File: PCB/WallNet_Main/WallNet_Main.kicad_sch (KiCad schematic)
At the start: 29 parts, among them J1 Conn_01x05_Pin, SW1 SW, U1 BT832

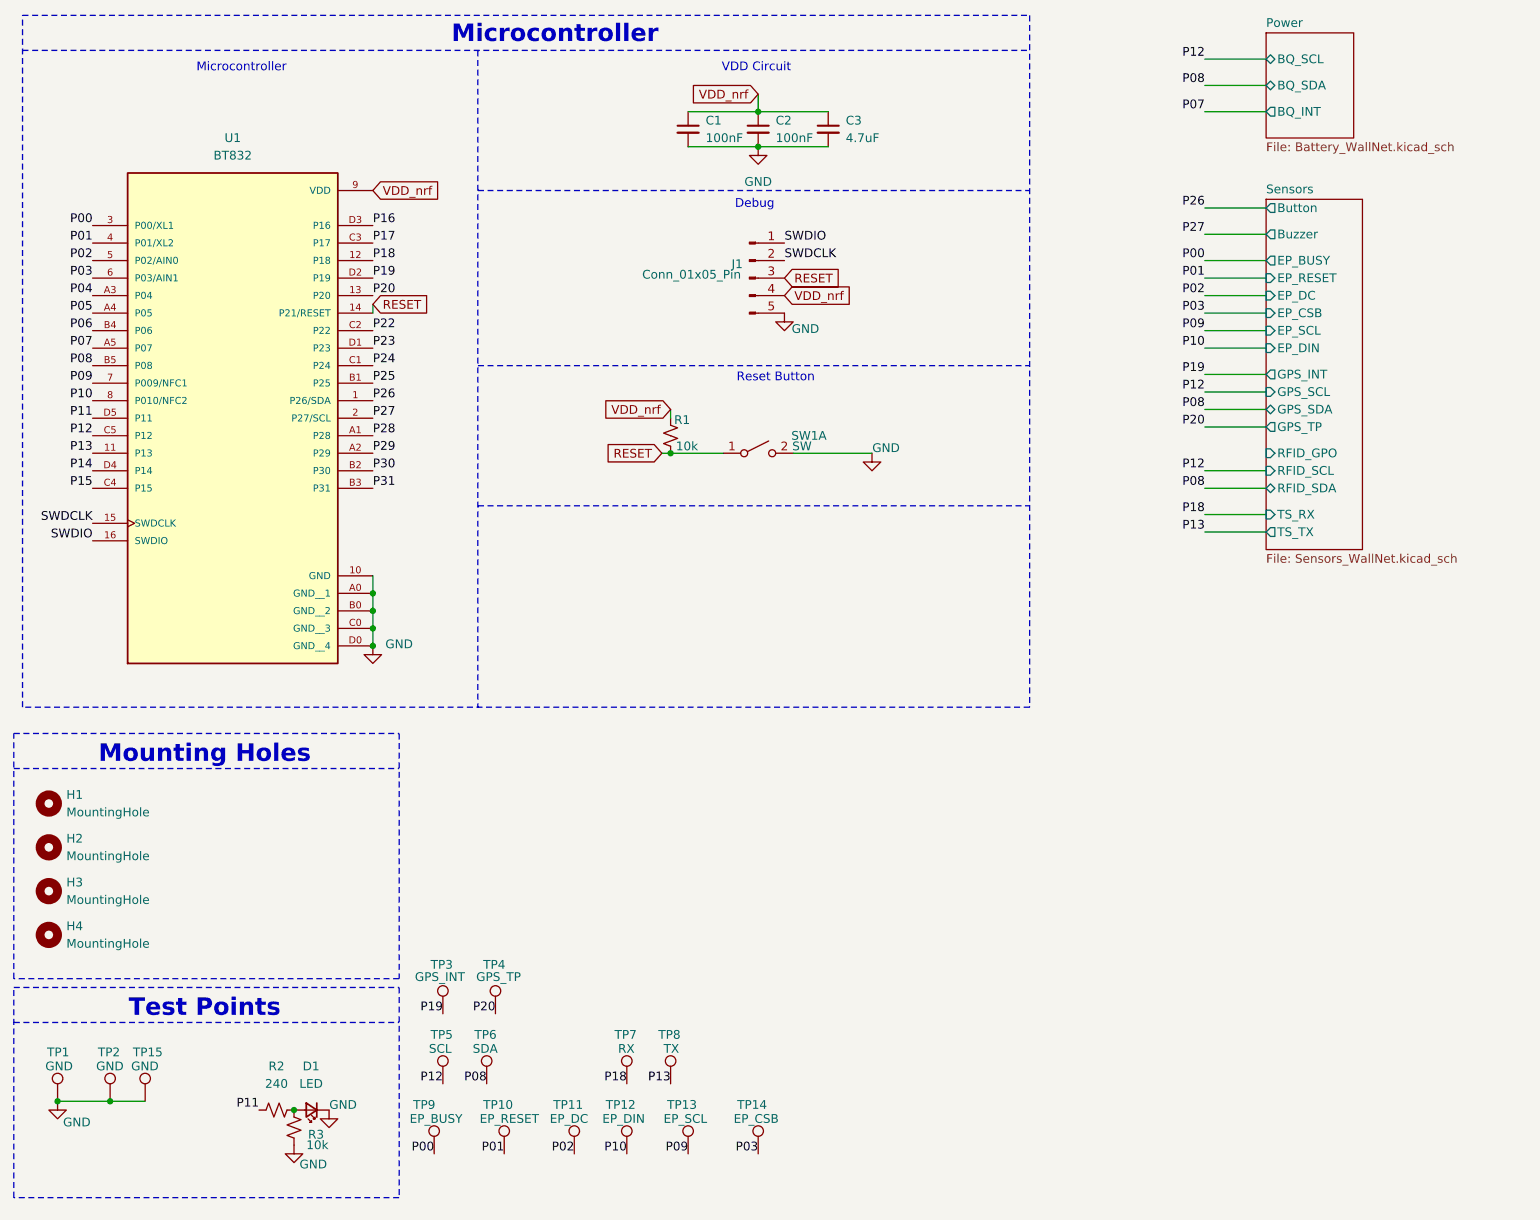
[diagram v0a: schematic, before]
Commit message: Implemented most changes
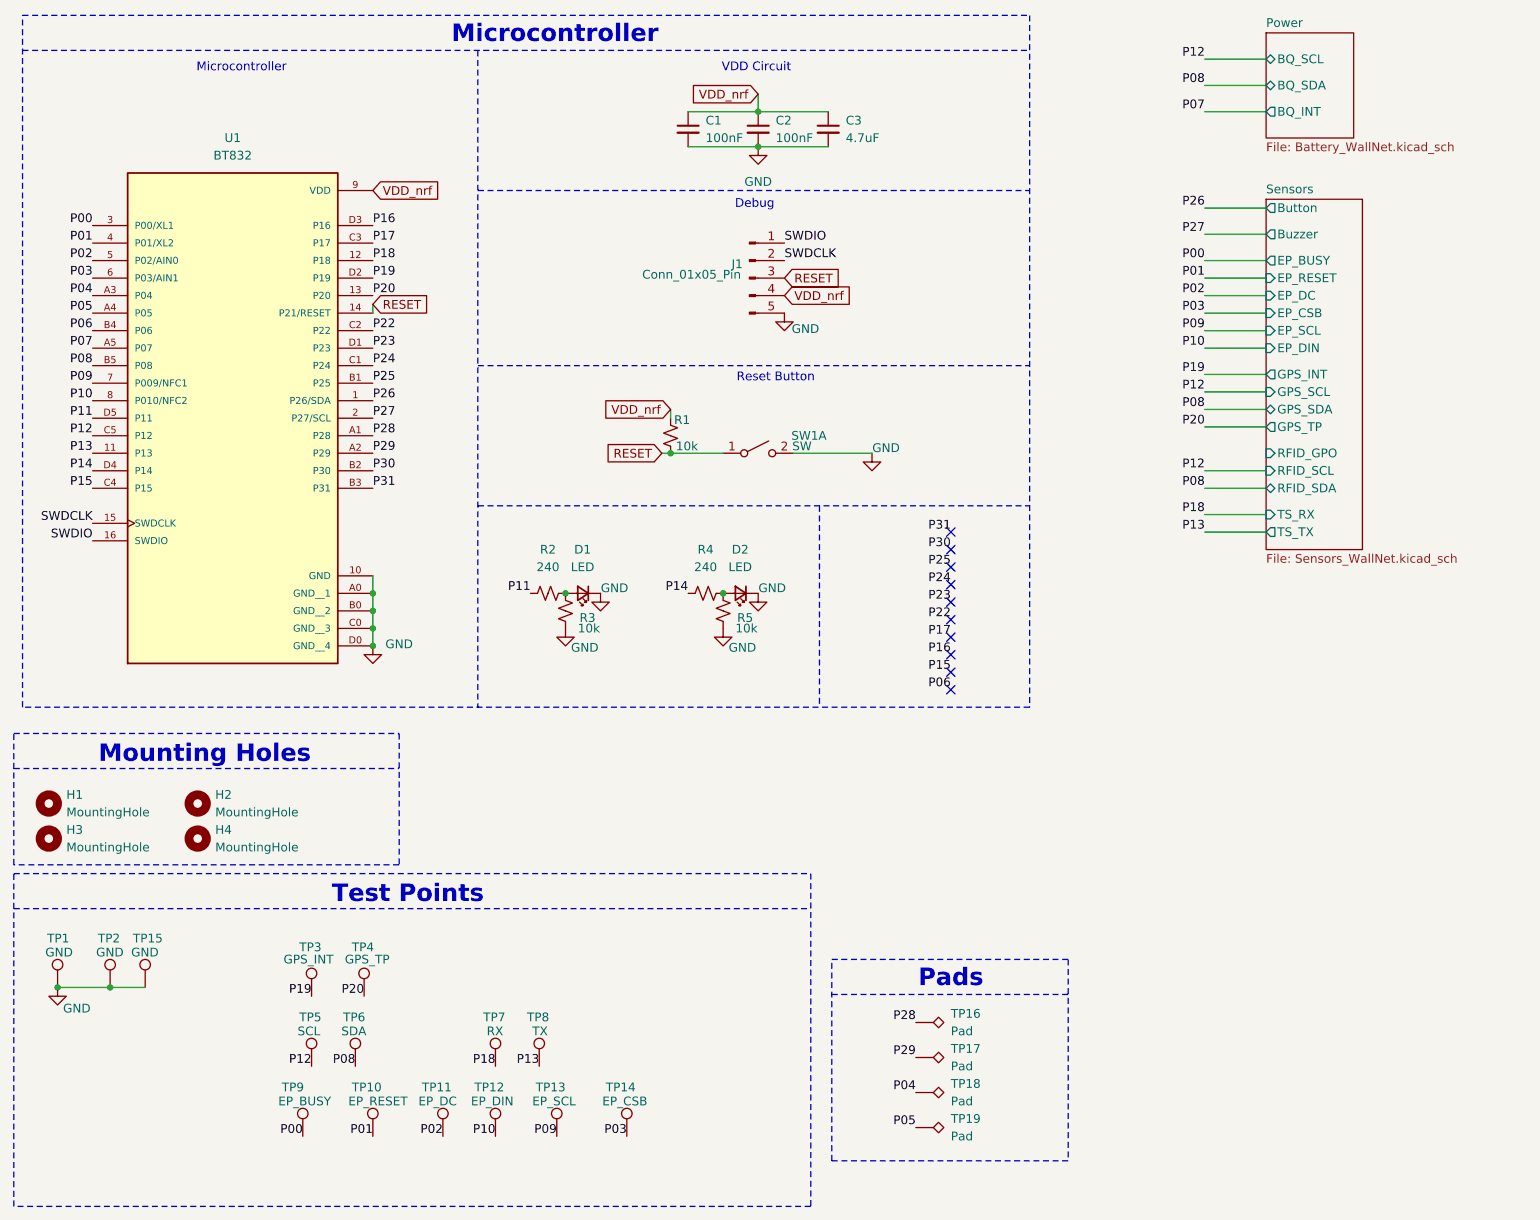
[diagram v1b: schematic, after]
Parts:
- added D2: LED, Diode_SMD:D_0603_1608Metric, symbol Device:LED_Small
- added R4: 240, Resistor_SMD:R_0603_1608Metric, symbol Device:R_Small_US
- added R5: 10k, Resistor_SMD:R_0603_1608Metric, symbol Device:R_Small_US
- added TP16, TP17, TP18, TP19: Pad, TestPoint:TestPoint_Pad_1.0x1.0mm, symbol Connector:TestPoint_Alt
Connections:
- net GND: now also D2.1 (K), R5.1
- net P04: now also TP18.1
- net P05: now also TP19.1
- net P14: now also R4.1
- net P28: now also TP16.1
- net P29: now also TP17.1
- new net: D2.2 (A), R4.2, R5.2
- no-connect marks 0 -> 10
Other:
- note added: "Pads"
- moved on the sheet: D1, H2, H3, H4, R2, R3, TP1, TP10, TP11, TP12, TP13, TP14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
